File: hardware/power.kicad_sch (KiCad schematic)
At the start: 42 parts, among them J5 B2B-EH-A, J6 Conn_01x02, J7 Conn_01x02, J8 Conn_01x02, J9 Conn_01x02, Q1 CSD25310Q2, U5 TPS63020DSJR, U6 BQ24074RGTR

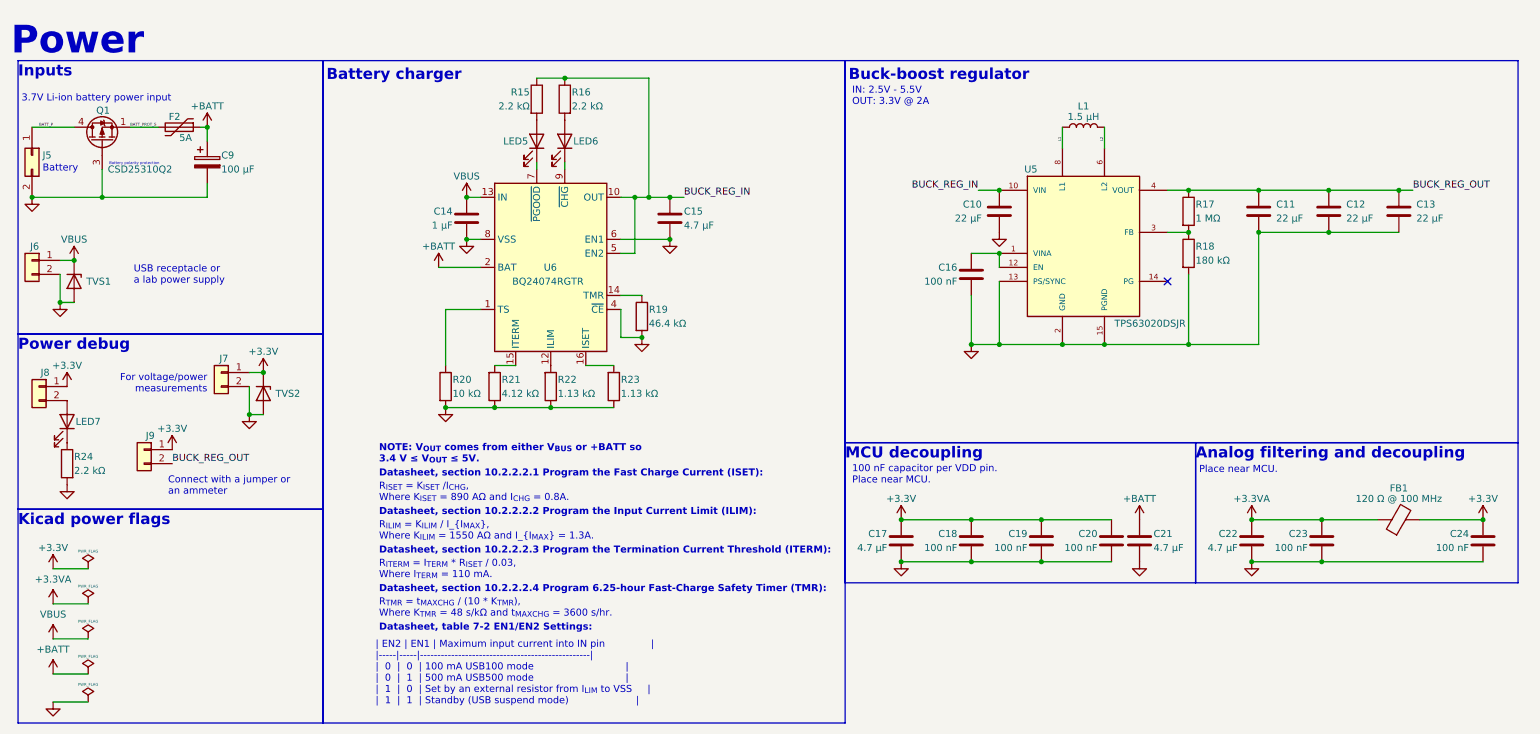
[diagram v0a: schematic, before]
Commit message: Start working on hw v4.0.0
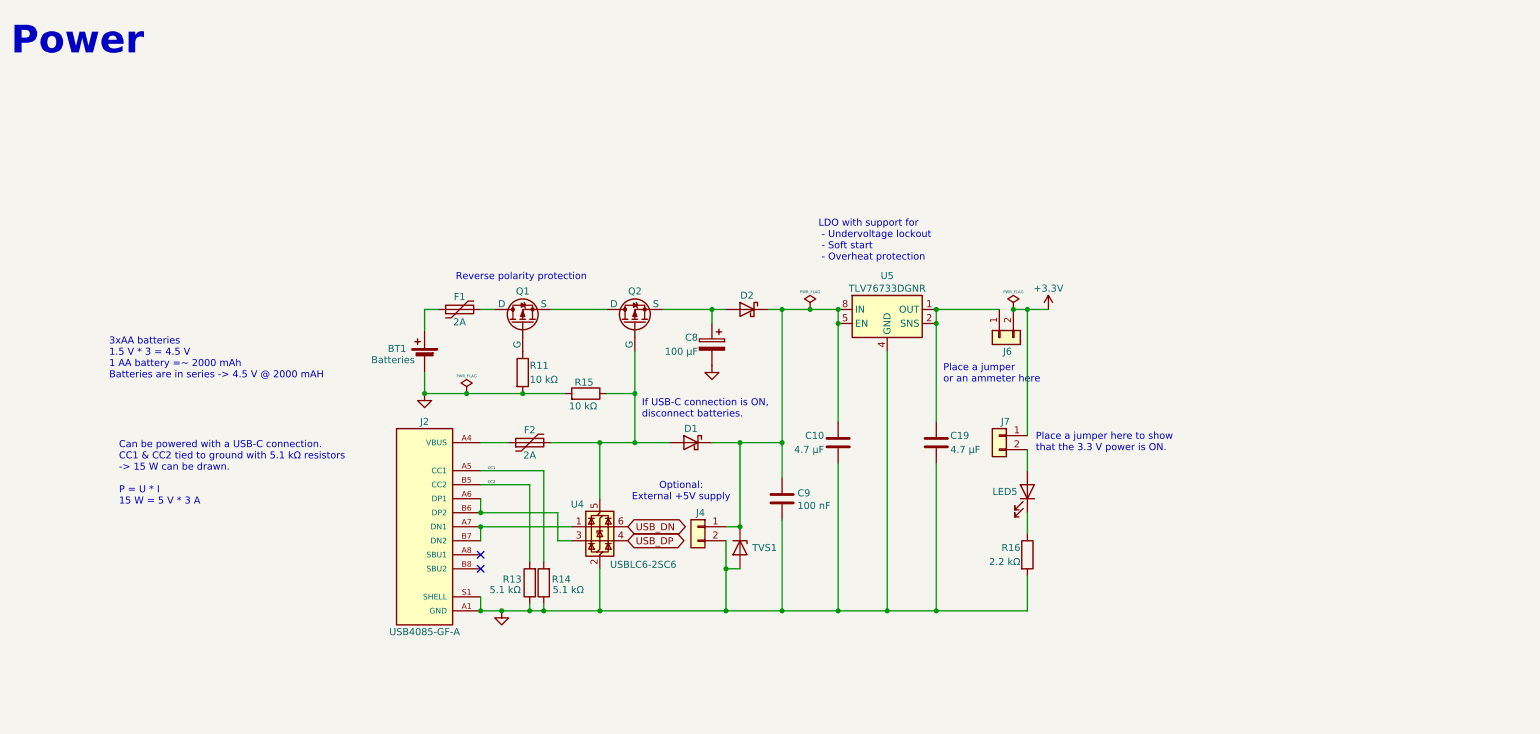
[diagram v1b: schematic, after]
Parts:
- removed C11, C12, C13: 22 µF, Capacitor_SMD:C_0805_2012Metric, symbol Device:C
- removed C14: 1 µF, Capacitor_SMD:C_0603_1608Metric, symbol Device:C
- removed C15, C17, C21, C22: 4.7 µF, Capacitor_SMD:C_0603_1608Metric, symbol Device:C
- removed C16, C18, C20, C23, C24: 100 nF, perfect_footprints:0402_1005_perfect, symbol Device:C
- removed C9: 100 µF, Capacitor_SMD:CP_Elec_5x5.3, symbol Device:C_Polarized
- removed FB1: 120 Ω @ 100 MHz, Resistor_SMD:R_0603_1608Metric, symbol Device:FerriteBead
- removed J5: B2B-EH-A, Connector_JST:JST_EH_B2B-EH-A_1x02_P2.50mm_Vertical, symbol Connector_Generic:Conn_02x01
- removed J8, J9: Conn_01x02, Connector_PinHeader_2.54mm:PinHeader_1x02_P2.54mm_Vertical, symbol Connector_Generic:Conn_01x02
- removed L1: 1.5 µH, Inductor_SMD:L_Taiyo-Yuden_NR-60xx, symbol Device:L
- removed LED6, LED7: LS T67K-K1L2-1-0-2-R18-Z, LED_SMD:LED_PLCC_2835, symbol Device:LED
- removed Q1: CSD25310Q2, Package_SON:Texas_DQK, symbol Transistor_FET:CSD25302Q2
- removed R17: 1 MΩ, perfect_footprints:0402_1005_perfect, symbol Device:R
- removed R18: 180 kΩ, perfect_footprints:0402_1005_perfect, symbol Device:R
- removed R19: 46.4 kΩ, perfect_footprints:0402_1005_perfect, symbol Device:R
- removed R20: 10 kΩ, perfect_footprints:0402_1005_perfect, symbol Device:R
- removed R21: 4.12 kΩ, perfect_footprints:0402_1005_perfect, symbol Device:R
- removed R22, R23: 1.13 kΩ, perfect_footprints:0402_1005_perfect, symbol Device:R
- removed R24: 2.2 kΩ, perfect_footprints:0402_1005_perfect, symbol Device:R
- removed TVS2: PE1605M1Q_R1_00001, Diode_SMD:D_0402_1005Metric, symbol Device:D_Zener
- removed U5: TPS63020DSJR, TPS63021DSJR:TPS63021DSJR, symbol TPS63021DSJR:TPS63021DSJR
- removed U6: BQ24074RGTR, Package_DFN_QFN:VQFN-16-1EP_3x3mm_P0.5mm_EP1.6x1.6mm, symbol BQ2407RGTR:BQ24074RGTR
- added BT1: Batteries, Battery:BatteryHolder_TruPower_BH-331P_3xAA, symbol Device:Battery_Cell
- added C8: 100 µF, Capacitor_SMD:CP_Elec_5x5.3, symbol Device:C_Polarized
- added C9: 100 nF, perfect_footprints:0402_1005_perfect, symbol Device:C
- added D1, D2: ~, symbol Device:D_Schottky
- added F1: 2A, symbol Device:Polyfuse
- added J2: USB4085-GF-A, USB4105-GF-A:USB4085-GF-A, symbol USB4085-GF-A:USB4085-GF-A
- added J4: Conn_01x02, Connector_PinHeader_2.54mm:PinHeader_1x02_P2.54mm_Vertical, symbol Connector_Generic:Conn_01x02
- added Q1, Q2: ~, symbol Simulation_SPICE:PMOS
- added R11: 10 kΩ, perfect_footprints:0402_1005_perfect, symbol Device:R
- added R13, R14: 5.1 kΩ, perfect_footprints:0402_1005_perfect, symbol Device:R
- added U4: USBLC6-2SC6, Package_TO_SOT_SMD:SOT-23-6, symbol Power_Protection:USBLC6-2SC6
- added U5: TLV76733DGNR, Package_SO:HVSSOP-8-1EP_3x3mm_P0.65mm_EP1.57x1.89mm_ThermalVias, symbol TLV76733DGNR:TLV76733DGNR
- C10: value 22 µF -> 4.7 µF; footprint Capacitor_SMD:C_0805_2012Metric -> Capacitor_SMD:C_0603_1608Metric; Digi-Key Part Number 1276-6526-1-ND -> 1276-1044-1-ND; Manufacturer Part Number CL21A226KOQNNNE -> CL10A475KP8NNNC
- C19: value 100 nF -> 4.7 µF; footprint perfect_footprints:0402_1005_perfect -> Capacitor_SMD:C_0603_1608Metric; Digi-Key Part Number 1276-1002-1-ND -> 1276-1044-1-ND; Manufacturer Part Number CL05B104KP5NNNC -> CL10A475KP8NNNC
- F2: value 5A -> 2A; footprint Fuse:Fuse_1812_4532Metric -> (none); Digi-Key Part Number 507-1781-1-ND -> (none); Manufacturer Bel Fuse Inc. -> (none); Manufacturer Part Number 0ZCG0300FF2B -> (none)
- R15: value 2.2 kΩ -> 10 kΩ; Digi-Key Part Number 311-2.20KLRCT-ND -> 311-10.0KLRCT-ND; Manufacturer Part Number RC0402FR-072K2L -> RC0402FR-0710KL
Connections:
- net +3.3V: now also J6.2 (Pin_2); no longer C19.1
- net GND: now also R15.2, R16.2, BT1.2 (-), C8.2, C9.1, J2.A1 (GND), J2.A12 (GND), J2.B1 (GND), J2.B12 (GND), J2.S1 (SHELL), J2.S2 (SHELL), J2.S3 (SHELL), J2.S4 (SHELL), J4.2 (Pin_2), R11.2, R13.1, R14.1, U4.2 (GND), U5.3 (NC), U5.4 (GND), U5.6 (GND), U5.9 (GND); no longer J6.2 (Pin_2), J7.2 (Pin_2)
- net at LED5.1 (K): now also R16.1
- net at LED5.2 (A): now also J7.2 (Pin_2); no longer R15.2
- net +BATT: no longer names the net of F2.1
- net +BATT: now also J2.A4 (VBUS), J2.A9 (VBUS), J2.B4 (VBUS), J2.B9 (VBUS)
- net BATT_PROT_S: no longer names the net of F2.2
- net BATT_PROT_S: now also R15.1, D1.2 (A), Q2.2 (G), U4.5 (VBUS)
- removed net BUCK_REG_IN: C10.1, R15.1, R16.1
- net VBUS: no longer names the net of J6.1 (Pin_1)
- net VBUS: now also C19.1, U5.1 (OUT), U5.2 (SNS); no longer TVS1.1 (K)
- new net: BT1.1 (+), F1.1
- new net: F1.2, Q1.1 (D)
- new net: C10.1, C9.2, D1.1 (K), D2.1 (K), J4.1 (Pin_1), TVS1.1 (K), U5.5 (EN), U5.8 (IN)
- new net: J2.A6 (DP1), J2.B6 (DP2), U4.3 (I/O2)
- new net: J2.A7 (DN1), J2.B7 (DN2), U4.1 (I/O1)
- new net: Q1.2 (G), R11.1
- new net: Q1.3 (S), Q2.1 (D)
- new net: C8.1, D2.2 (A), Q2.3 (S)
- new net CC1: J2.A5 (CC1), R14.2
- new net CC2: J2.B5 (CC2), R13.2
- new net USB_DN: U4.6 (I/O1)
- new net USB_DP: U4.4 (I/O2)
- no-connect marks 1 -> 2
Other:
- note added: "3xAA batteries 1.5 V * 3 = 4.5 V 1 AA battery =~ 2000 mAh Batteries are in series -> 4.5 V @ 2000 mAH"
- note added: "Can be powered with a USB-C connection. CC1 & CC2 tied to ground with 5.1 kΩ resistors -> 15 W can be drawn. P = U * I 15 W = 5 V * 3 A"
- note added: "If USB-C connection is ON, disconnect batteries."
- note added: "LDO with support for - Undervoltage lockout - Soft start - Overheat protection"
- note added: "Optional: External +5V supply"
- note added: "Place a jumper here to show that the 3.3 V power is ON."
- note added: "Place a jumper or an ammeter here"
- note added: "Reverse polarity protection"
- note removed: "100 nF capacitor per VDD pin. Place near MCU."
- note removed: "3.7V Li-ion battery power input"
- note removed: "Analog filtering and decoupling"
- note removed: "Battery"
- note removed: "Battery charger"
- note removed: "Battery polarity protection"
- note removed: "Buck-boost regulator"
- note removed: "Connect with a jumper or an ammeter"
- note removed: "Datasheet, section 10.2.2.2.1 Program the Fast Charge Current (ISET):"
- note removed: "Datasheet, section 10.2.2.2.2 Program the Input Current Limit (ILIM):"
- note removed: "Datasheet, section 10.2.2.2.3 Program the Termination Current Threshold (ITERM):"
- note removed: "Datasheet, section 10.2.2.2.4 Program 6.25-hour Fast-Charge Safety Timer (TMR):"
- note removed: "Datasheet, table 7-2 EN1/EN2 Settings:"
- note removed: "For voltage/power measurements"
- note removed: "IN: 2.5V - 5.5V OUT: 3.3V @ 2A"
- note removed: "Inputs"
- note removed: "Kicad power flags"
- note removed: "MCU decoupling"
- note removed: "NOTE: V_{OUT} comes from either V_{BUS} or +BATT so 3.4 V ≤ V_{OUT} ≤ 5V."
- note removed: "Place near MCU."
- note removed: "Power debug"
- note removed: "R_{ILIM} = K_{ILIM} / I_{I_{MAX}}, Where K_{ILIM} = 1550 AΩ and I_{I_{MAX}} = 1.3A."
- note removed: "R_{ISET} = K_{ISET} /I_{CHG}, Where K_{ISET} = 890 AΩ and I_{CHG} = 0.8A."
- note removed: "R_{ITERM} = I_{TERM} * R_{ISET} / 0.03, Where I_{TERM} = 110 mA."
- note removed: "R_{TMR} = t_{MAXCHG} / (10 * K_{TMR}), Where K_{TMR} = 48 s/kΩ and t_{MAXCHG} = 3600 s/hr."
- note removed: "USB receptacle or a lab power supply"
- note removed: "| EN2 | EN1 | Maximum input current into IN pin | |-----|-----|-------------------------------------------------| | 0 | 0 | 100 mA USB100 mode | | 0 | 1 | 500 mA USB500 mode | | 1 | 0 | Set by an external resistor from I_{LIM} to VSS | | 1 | 1 | Standby (USB suspend mode) |"
